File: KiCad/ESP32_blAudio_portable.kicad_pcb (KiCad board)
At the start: 2 copper layers, 90 x 75 mm, 102 parts, among them J1 Conn_01x15_Male, J2 Conn_01x15_Male, J3 Conn_01x02_Male, J4 Conn_01x02_Male, J5 Conn_01x02_Male, J6 ASJ-99H, J7 Conn_01x16_Female, SW1 TS02, SW2 TS02, SW3 TS02, SW4 PEC12R, SW5 TS02, U1 MCP73831-2-OT, U2 TFA9879HN, U3 TFA9879HN, U4 AK5720VT, U5 AP3012, U6 PCF8574

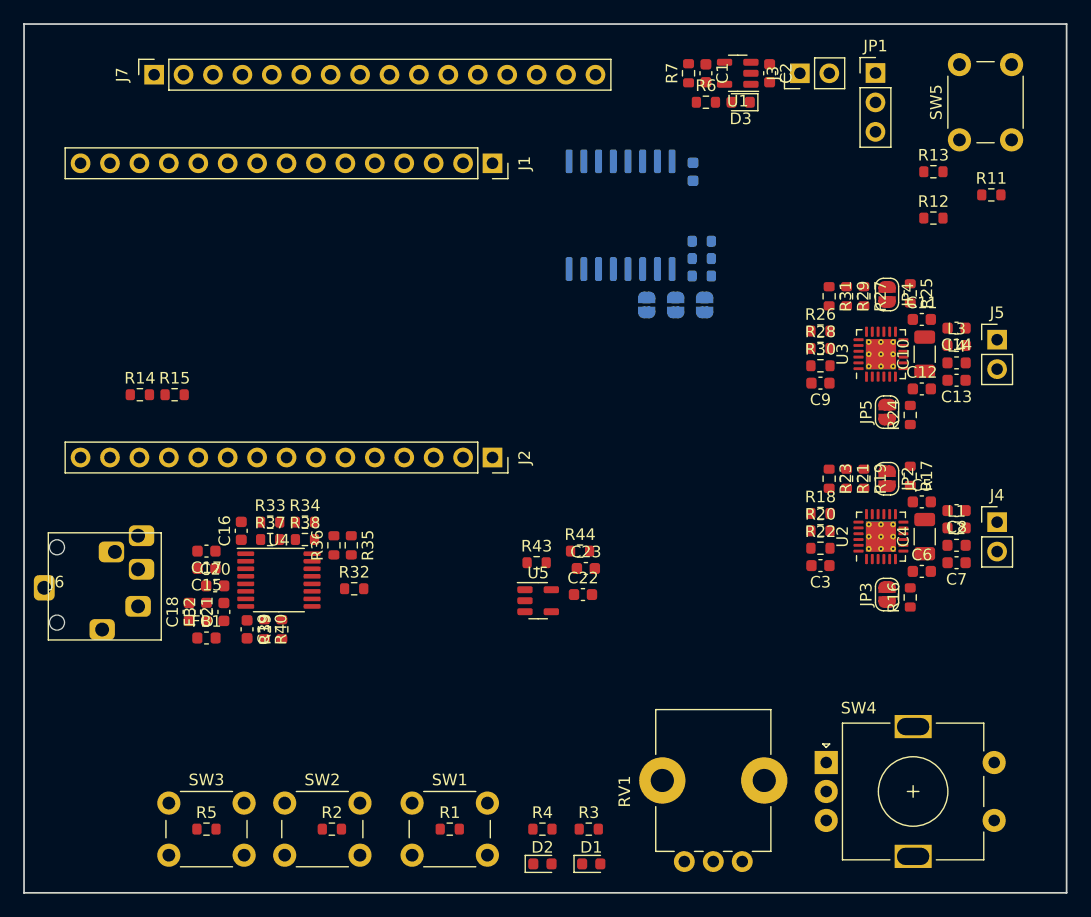
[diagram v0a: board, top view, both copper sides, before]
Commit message: -layout work
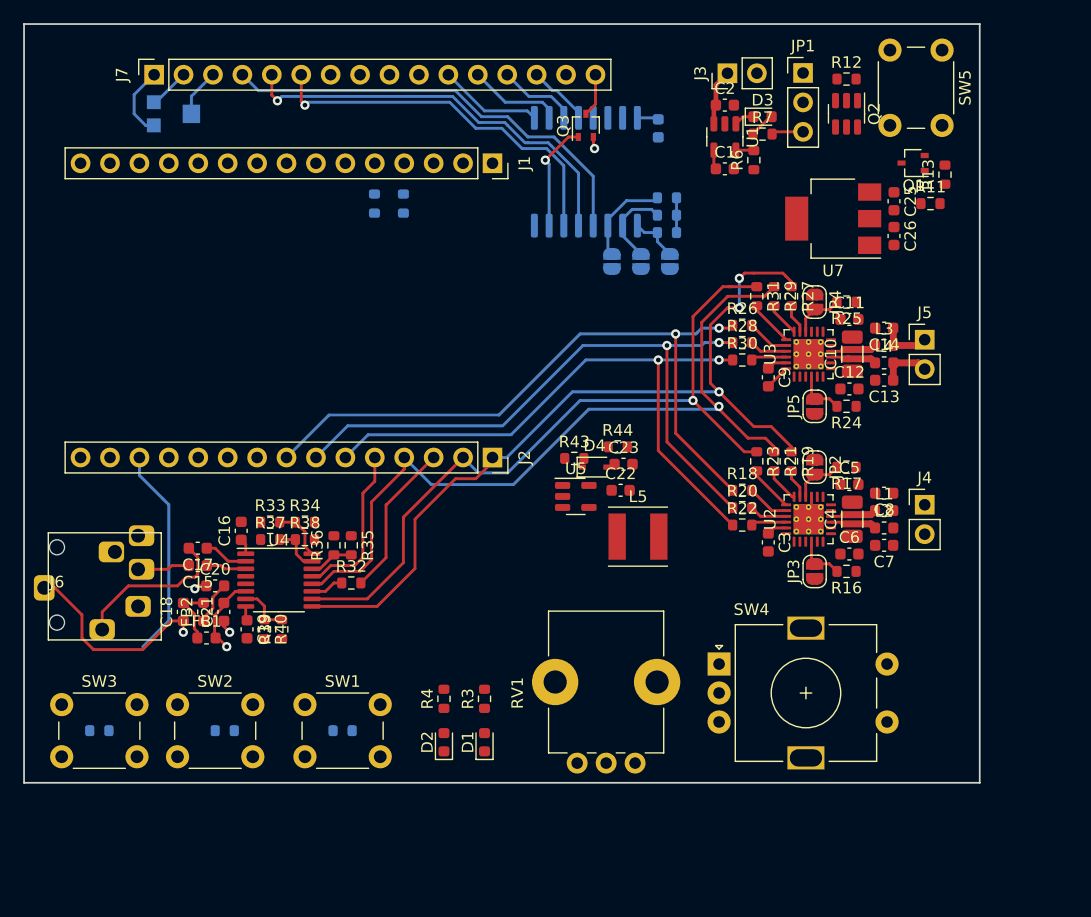
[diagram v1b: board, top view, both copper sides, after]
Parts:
- added C25: 1u, Capacitor_SMD:C_0603_1608Metric, F.Cu at (126.1, 36.3)
- added C26: 1u, Capacitor_SMD:C_0603_1608Metric, F.Cu at (126.1, 39.3)
- added D4: 30V 1A, Diode_SMD:D_SOD-323, F.Cu at (100.2, 59.2)
- added L5: 33u, Inductor_SMD:L_Taiyo-Yuden_NR-50xx, F.Cu at (104.0, 65.2)
- added Q1: 2N7002, Package_TO_SOT_SMD:SOT-323_SC-70, F.Cu at (127.8, 33.0)
- added Q2: Q_PMOS_DGS, Package_TO_SOT_SMD:SOT-23-6, F.Cu at (122.0, 28.8)
- added Q3: 2N7002, Package_TO_SOT_SMD:SOT-323_SC-70, F.Cu at (99.5, 29.8)
- added RV2: TC33X_10k, Custom:trimmer_Bourns_tc33x, B.Cu at (64.0, 28.8)
- added U7: NCP1117-3.3_SOT223, Package_TO_SOT_SMD:SOT-223-3_TabPin2, F.Cu at (120.8, 37.8)
- R1, R14, R15, R2, R5: moved to B.Cu
- moved R14 26.1 mm to (81.2, 36.5), turned to 90 degrees
- moved R15 25.7 mm to (83.8, 36.5), turned to 90 degrees
- moved R3 14.4 mm to (90.8, 79.2), turned to 90 degrees
- moved R12 14.2 mm to (122.0, 25.8)
- moved R4 14.1 mm to (87.2, 79.2), turned to 90 degrees
- moved D1 14.0 mm to (90.8, 83.0), turned to 90 degrees
- moved D2 13.5 mm to (87.2, 83.0), turned to 90 degrees
- moved R1 12.6 mm to (78.5, 82.0), turned to 180 degrees
- moved R2 12.6 mm to (68.3, 82.0), turned to 180 degrees
- moved R5 12.6 mm to (57.5, 82.0), turned to 180 degrees
- moved RV1 12.6 mm to (103.8, 84.8)
- moved SW1 12.6 mm to (75.2, 79.8)
- moved SW2 12.6 mm to (64.2, 79.8)
- moved SW3 12.6 mm to (54.2, 79.8)
- moved SW4 12.6 mm to (111.0, 76.2)
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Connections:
- C22 pad 1: +3V3 -> +VDC
- J1 pad 1: unconnected-(J1-Pad1) -> +3V3
- J1 pad 2: unconnected-(J1-Pad2) -> /PWR_ON
- J1 pad 3: unconnected-(J1-Pad3) -> /EN_5V
- J1 pad 4: unconnected-(J1-Pad4) -> /SCL
- J1 pad 5: unconnected-(J1-Pad5) -> /SDA
- J1 pad 6: unconnected-(J1-Pad6) -> /ENC_SW
- J1 pad 7: unconnected-(J1-Pad7) -> /ENC_A
- J1 pad 8: unconnected-(J1-Pad8) -> /ENC_B
- J1 pad 9: unconnected-(J1-Pad9) -> /ANA_VOL
- J2 pad 10: unconnected-(J2-Pad10) -> /LED2
- J2 pad 11: unconnected-(J2-Pad11) -> /BTTN1
- J2 pad 12: unconnected-(J2-Pad12) -> /BTTN2
- J2 pad 13: unconnected-(J2-Pad13) -> /BTTN3
- J2 pad 15: unconnected-(J2-Pad15) -> +3V3
- J2 pad 6: unconnected-(J2-Pad6) -> /LRCK1
- J2 pad 7: unconnected-(J2-Pad7) -> /SCK1
- J2 pad 8: unconnected-(J2-Pad8) -> /SDI1
- J2 pad 9: unconnected-(J2-Pad9) -> /LED1
- U5 pad 5: +3V3 -> +VDC
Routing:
- net /SDI2: track 0.00 -> 71.6 mm, vias 0 -> 3
- net /SCK2: track 0.00 -> 69.3 mm, vias 0 -> 1
- net /LRCK2: track 0.00 -> 64.8 mm, vias 0 -> 1
- net /SDI1: track 0.00 -> 58.8 mm, vias 0 -> 2
- net /SCK1: track 0.00 -> 56.4 mm, vias 0 -> 2
- net /LRCK1: track 0.00 -> 53.8 mm, vias 0 -> 2
- net /Display/LCD_RS: track 0.00 -> 38.2 mm
- net /Display/LCD_R/~{W}: track 0.00 -> 36.0 mm, vias 0 -> 1
- net /Display/LCD_E: track 0.00 -> 32.6 mm, vias 0 -> 1
- net GND: track 0.00 -> 31.1 mm, vias 0 -> 4
- net /BTTN3: track 0.00 -> 18.3 mm
- net +3V3: track 0.00 -> 15.3 mm, vias 0 -> 1
- net /~{PDN}: track 0.00 -> 14.1 mm
- net Net-(C17-Pad2): track 0.00 -> 13.7 mm
- net /MCLK: track 0.00 -> 13.5 mm
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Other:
- board size 90 x 75 mm -> 82.5 x 65.5 mm
